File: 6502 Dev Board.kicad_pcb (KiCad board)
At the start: 2 copper layers, 158.8 x 134.6 mm, 827 parts, among them J1 Barrel_Jack, J2 Signals, J3 Addresses, J4 Data, SW1 Power, SW2 Reset, U1 W65C02S, U2 62256, U3 L7805, U4 DS1233, U5 28C256, U6 GAL22V10, X1 1.8432

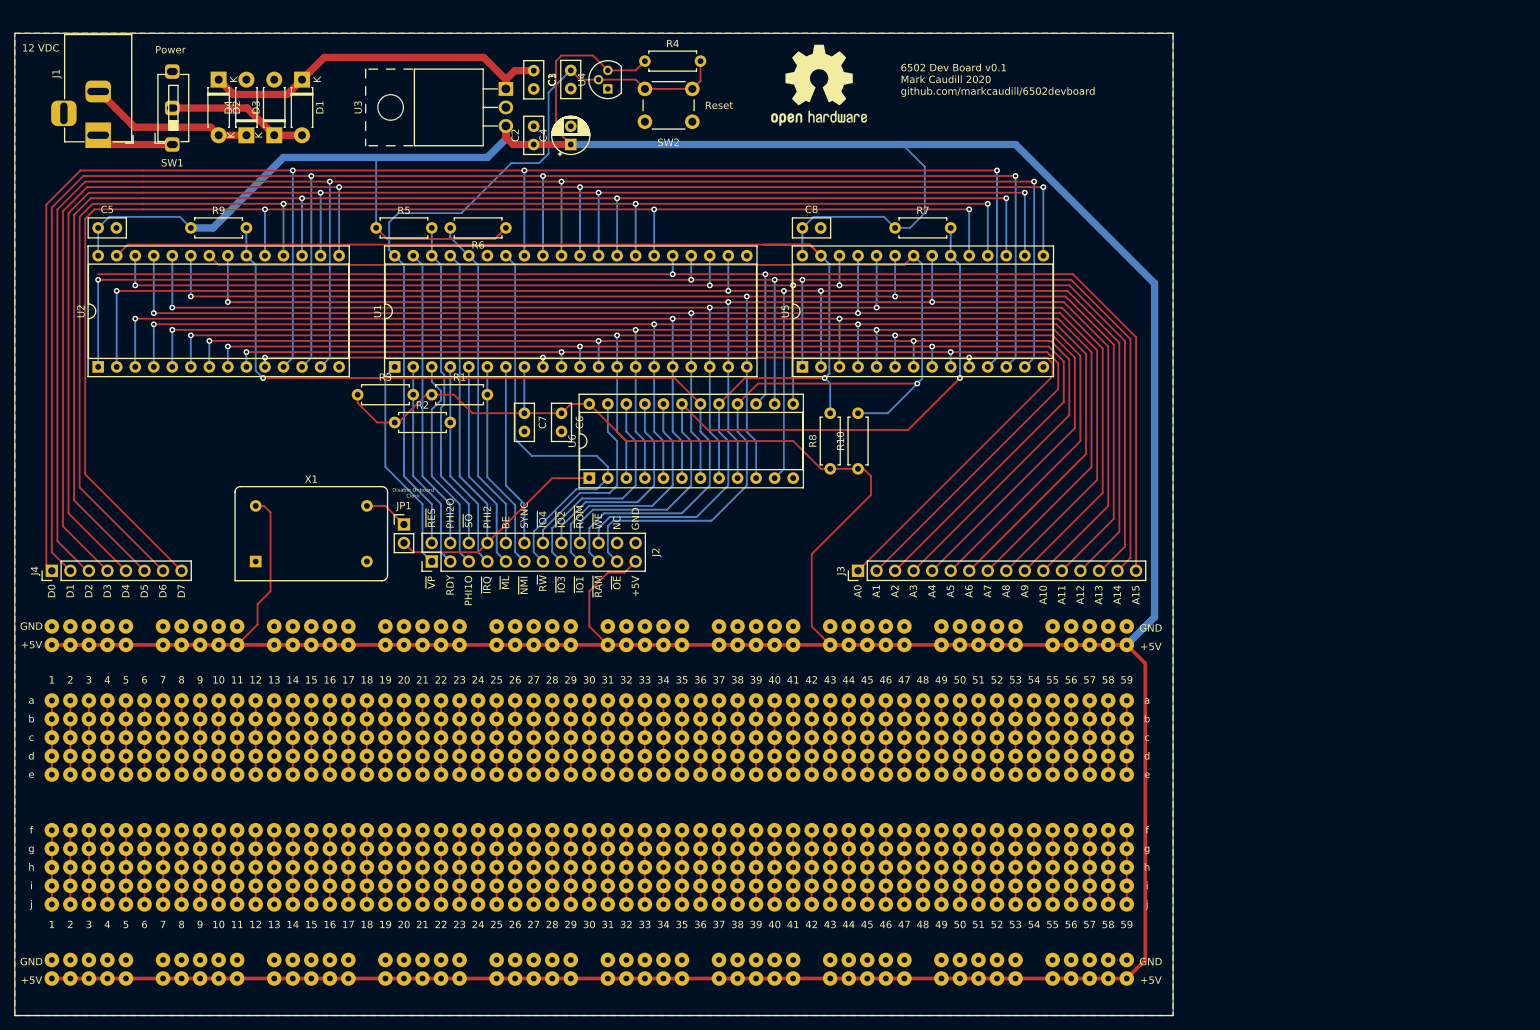
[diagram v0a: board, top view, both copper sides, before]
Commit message: Update metadata.
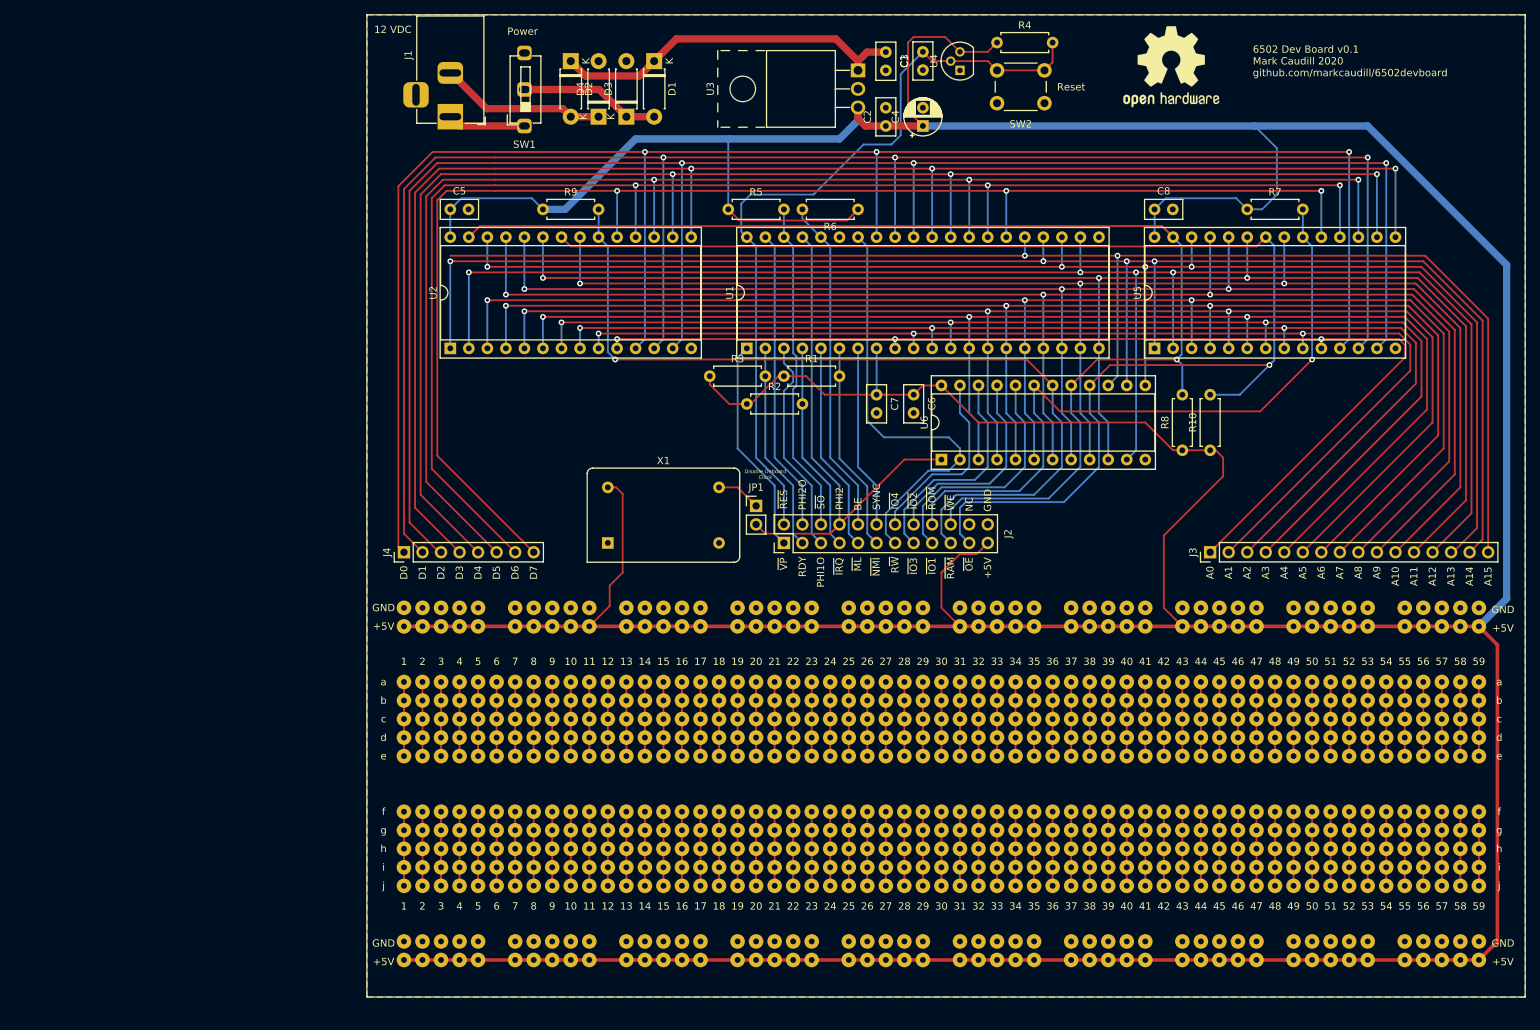
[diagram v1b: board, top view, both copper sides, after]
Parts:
- moved REF** 48.3 mm to (201.9, 139.7)
- moved REF** 48.3 mm to (201.9, 144.8)
- moved REF** 48.3 mm to (181.6, 134.6)
- moved REF** 48.3 mm to (191.8, 144.8)
- moved REF** 48.3 mm to (163.8, 144.8)
- moved REF** 48.3 mm to (209.6, 139.7)
- moved REF** 48.3 mm to (163.8, 139.7)
- moved REF** 48.3 mm to (209.6, 144.8)
- moved REF** 48.3 mm to (184.2, 139.7)
- moved REF** 48.3 mm to (191.8, 137.2)
- moved REF** 48.3 mm to (181.6, 137.2)
- moved REF** 48.3 mm to (201.9, 152.4)
- moved REF** 48.3 mm to (184.2, 134.6)
- moved REF** 48.3 mm to (191.8, 142.2)
- moved REF** 48.3 mm to (181.6, 139.7)
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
